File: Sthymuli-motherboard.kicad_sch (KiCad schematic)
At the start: 284 parts, among them J1 USB_C_Receptacle_USB2.0_16P, J2 Conn_01x09, J3 Conn_01x03, J4 Conn_01x06, Q1 Q_NMOS_Depletion_GSD, Q10 NX7002AK, Q11 NX7002AK, Q12 NX7002AK, Q13 NX7002AK, Q14 NX7002AK, Q15 NX7002AK, Q2 Q_NMOS_Depletion_GSD, Q3 Q_NMOS_Depletion_GSD, Q4 Q_NMOS_Depletion_GSD, Q5 Q_NMOS_Depletion_GSD, Q6 Q_NMOS_Depletion_GSD, Q7 PMOS, Q8 NX7002AK, Q9 NX7002AK, SW1 SW_Push, SW10 SW_Push, SW2 SW_Push, SW3 SW_Push, SW4 SW_Push, SW5 SW_Push, SW6 SW_Push, SW7 SW_Push, SW8 SW_Push, SW9 SW_Push, U1 ESP32-S3-WROOM-1, U10 74HC4051, U11 MCP6L01x-xOT, U12 74HC4051, U13 LSM6DS3, U14 LSM6DS3, U15 ITR9909, U16 ITR9909, U17 ITR9909, U18 ITR9909, U19 ITR9909, U2 AP2112K-3.3, U20 ITR9909, U21 ITR9909, U22 ITR9909, U3 BQ76905RGRR, U4 AP62300WU, U5 BQ25713, U6 AP62300WU, U7 MCP23017_SO, U8 AP22913CN4, U9 IRM-H6xxT

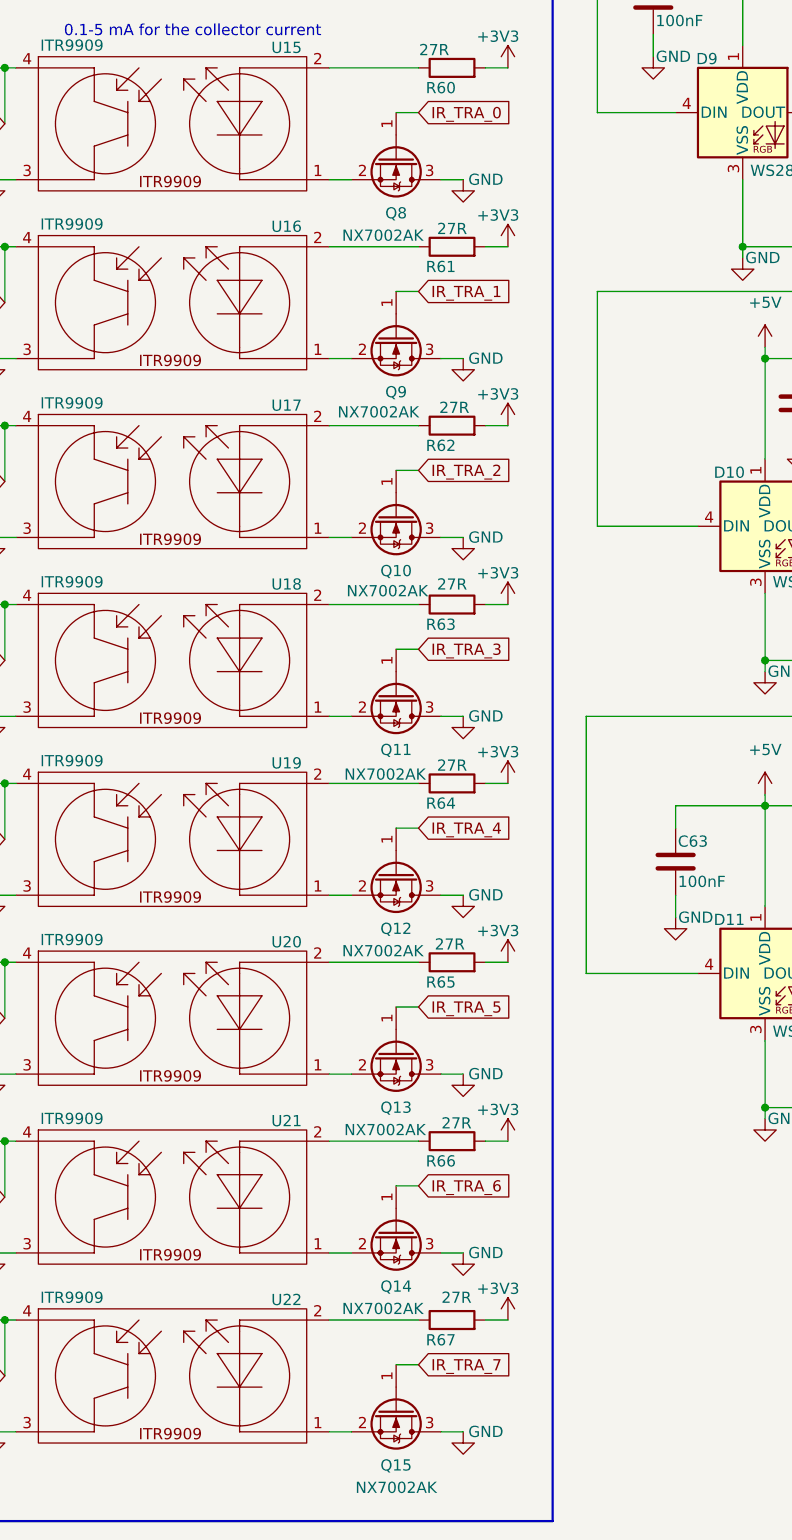
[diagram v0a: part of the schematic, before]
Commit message: added footprint
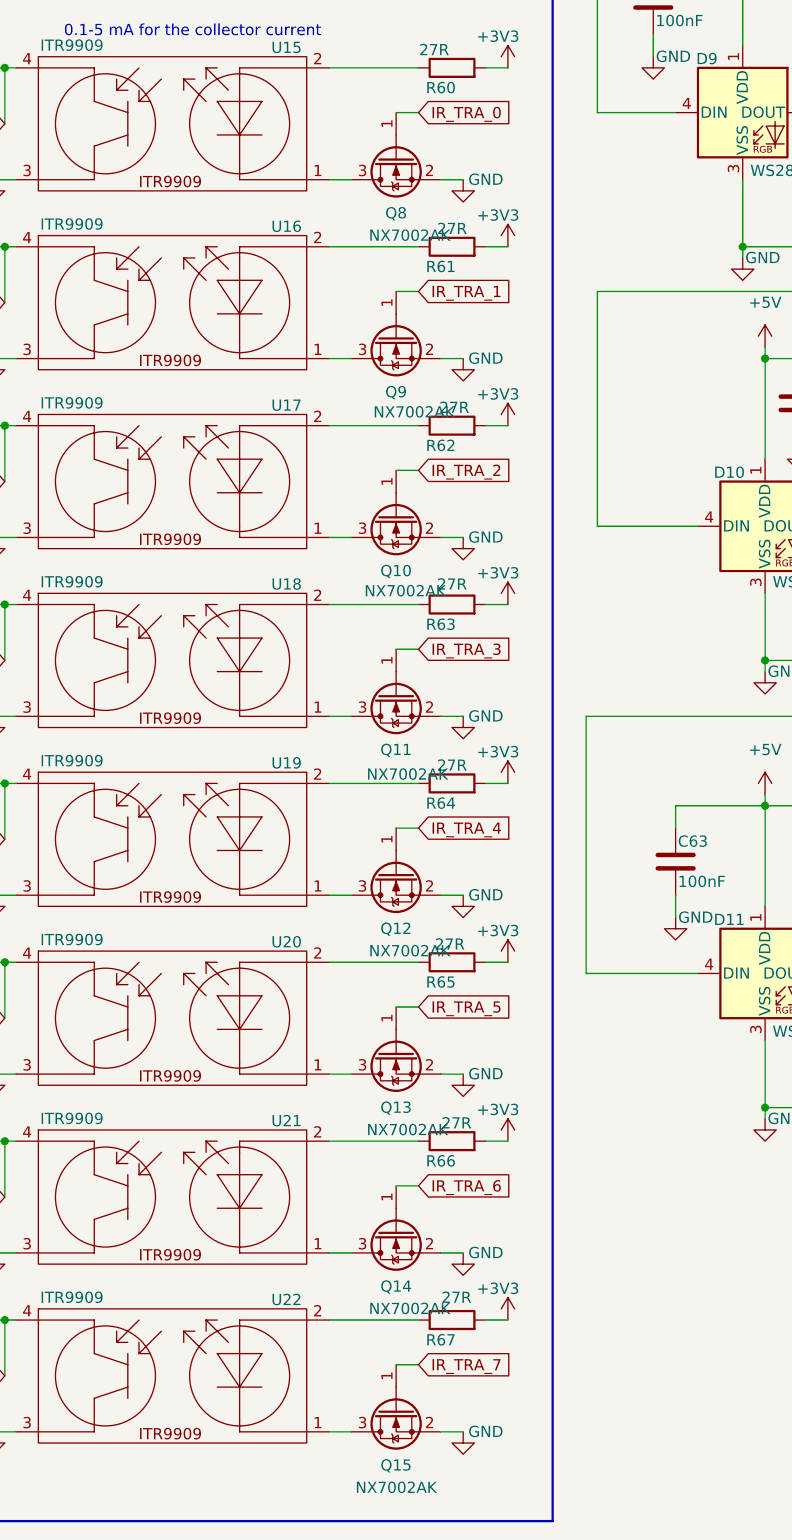
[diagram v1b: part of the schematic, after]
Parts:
- BT1, BT2, BT3, BT4: footprint (none) -> sthymuli:Battery_Holder_18650_robop
- D1, D12, D2, D3, D4, D5, D6: footprint (none) -> Diode_SMD:D_SOD-123F
- ES1: footprint (none) -> Package_DFN_QFN:QFN-28-1EP_4x4mm_P0.45mm_EP2.4x2.4mm
- F1, F2, F3, F4: footprint (none) -> Resistor_SMD:R_0805_2012Metric
- J1: footprint (none) -> Connector_USB:USB_C_Receptacle_G-Switch_GT-USB-7010ASV
- J2: footprint (none) -> Connector_PinHeader_2.54mm:PinHeader_1x09_P2.54mm_Vertical
- J3: footprint (none) -> Connector_PinHeader_2.54mm:PinHeader_1x03_P2.54mm_Vertical
- Q1, Q2, Q3, Q4, Q5, Q6, Q7: footprint (none) -> Package_SON:VSON-8_3.3x3.3mm_P0.65mm_NexFET
- Q10, Q11, Q12, Q13, Q14, Q15, Q8, Q9: footprint (none) -> Package_TO_SOT_SMD:SOT-23
- SW1, SW10, SW2, SW3, SW4, SW5, SW6, SW7, SW8, SW9: footprint (none) -> sthymuli:XKB5858
- TH1: footprint (none) -> Resistor_SMD:R_0603_1608Metric
- U15, U16, U17, U18: footprint (none) -> sthymuli:ITR_9909_Horizontal
- U19, U20, U21, U22: footprint (none) -> sthymuli:ITR_9909_Vertical
- U3: footprint BQ76905RGRR:IC_BQ76905RGRR -> Package_DFN_QFN:Texas_RGP0020H_VQFN-20-1EP_4x4mm_P0.5mm_EP2.4x2.4mm
- U5: footprint (none) -> Package_DFN_QFN:QFN-32-1EP_4x4mm_P0.4mm_EP2.9x2.9mm
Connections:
- net GND: now also Q10.2 (S), Q11.2 (S), Q12.2 (S), Q13.2 (S), Q14.2 (S), Q15.2 (S), Q8.2 (S), Q9.2 (S); no longer Q10.3 (D), Q11.3 (D), Q12.3 (D), Q13.3 (D), Q14.3 (D), Q15.3 (D), Q8.3 (D), Q9.3 (D)
- net at U16.1: now also Q9.3 (D); no longer Q9.2 (S)
- net at U20.1: now also Q13.3 (D); no longer Q13.2 (S)
- net at U22.1: now also Q15.3 (D); no longer Q15.2 (S)
- net at U15.1: now also Q8.3 (D); no longer Q8.2 (S)
- net at U18.1: now also Q11.3 (D); no longer Q11.2 (S)
- net at U21.1: now also Q14.3 (D); no longer Q14.2 (S)
- net at U17.1: now also Q10.3 (D); no longer Q10.2 (S)
- net at U19.1: now also Q12.3 (D); no longer Q12.2 (S)
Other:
- moved on the sheet: Q10, Q11, Q12, Q13, Q14, Q15, Q8, Q9

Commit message: started layout of component
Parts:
- removed C102, C63, C72, C78, C82, C86, C90, C96: 100nF, Capacitor_SMD:C_0402_1005Metric, symbol Device:C
- removed D11, D16, D20, D24, D28, D32, D36, D40: WS2812B, LED_SMD:LED_WS2812B_PLCC4_5.0x5.0mm_P3.2mm, symbol LED:WS2812B
- J4: footprint (none) -> sthymuli:ConnectorSpring
- L1: footprint (none) -> sthymuli:FHD4020S-2R2MT
- L2, L3: footprint (none) -> sthymuli:FXL0630-3R3-M
- L4: footprint (none) -> sthymuli:TDK VFS5045VA301
- LS1: footprint (none) -> sthymuli:Speaker KELIKING KLJ-01304T-08R07W
- MKTD4015BPN1: footprint (none) -> sthymuli:SAMZO MIC-4013-G-G00

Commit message: fixed some footprint issue, advanced layout
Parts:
- added C2: 100nF, Capacitor_SMD:C_0402_1005Metric, symbol Device:C
- added D2: WS2812B, LED_SMD:LED_WS2812B_PLCC4_5.0x5.0mm_P3.2mm, symbol LED:WS2812B
- C49: renamed from C27; footprint Capacitor_SMD:C_0402_1005Metric -> Capacitor_SMD:C_0805_2012Metric
- C50: renamed from C28; footprint Capacitor_SMD:C_0402_1005Metric -> Capacitor_SMD:C_0805_2012Metric
- C51: renamed from C29; footprint Capacitor_SMD:C_0402_1005Metric -> Capacitor_SMD:C_0805_2012Metric
- C72: renamed from C50; footprint Capacitor_SMD:C_0805_2012Metric -> Capacitor_SMD:C_0402_1005Metric
- C76: renamed from C54; footprint Capacitor_SMD:C_0805_2012Metric -> Capacitor_SMD:C_0402_1005Metric
- C81: renamed from C59; footprint Capacitor_SMD:C_0402_1005Metric -> Capacitor_SMD:C_0805_2012Metric
- renumbered C65 to C1, C62 to C10, C70 to C11, C76 to C12, C80 to C13, C84 to C14, C88 to C15, C94 to C16, C100 to C17, C68 to C18, C71 to C19, C77 to C20, C81 to C21, C85 to C22, C89 to C23, C95 to C24, C101 to C25, C4 to C26, C5 to C27, C6 to C28, C7 to C29, C74 to C3, C8 to C30, C9 to C31, C10 to C32, C11 to C33, C12 to C34, C13 to C35, C14 to C36, C15 to C37, C16 to C38, C17 to C39, C79 to C4, C18 to C40, C19 to C41, C20 to C42, C21 to C43, C22 to C44, C23 to C45, C24 to C46, C25 to C47, C26 to C48, C83 to C5, C30 to C52, C31 to C53, C32 to C54, C33 to C55, C34 to C56, C35 to C57, C36 to C58, C37 to C59, C87 to C6, C38 to C60, C39 to C61, C40 to C62, C41 to C63, C42 to C64, C43 to C65, C44 to C66, C45 to C67, C46 to C68, C47 to C69, C92 to C7, C48 to C70, C49 to C71, C51 to C73, C52 to C74, C53 to C75, C55 to C77, C56 to C78, C57 to C79, C98 to C8, C58 to C80, C60 to C82, C61 to C83, C64 to C84, C66 to C85, C67 to C86, C69 to C87, C73 to C88, C75 to C89, C104 to C9, C91 to C90, C93 to C91, C97 to C92, C99 to C93, C103 to C94, C105 to C95, C1 to C96, C2 to C97, C3 to C98, D13 to D1, D9 to D10, D14 to D11, D18 to D12, D22 to D13, D26 to D14, D30 to D15, D34 to D16, D38 to D17, D10 to D18, D15 to D19, D19 to D20, D23 to D21, D27 to D22, D31 to D23, D35 to D24, D39 to D25, D1 to D26, D2 to D27, D3 to D28, D4 to D29, D17 to D3, D5 to D30, D6 to D31, D7 to D32, D8 to D33, D12 to D34, D21 to D4, D25 to D5, D29 to D6, D33 to D7, D37 to D8, D41 to D9
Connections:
- net +5V: now also C2.1, D2.1 (VDD)
- net +BATT: now also D26.1 (K); no longer BT1.1 (+)
- net GND: now also C2.2, D2.3 (VSS)
- net at BT1.2 (-), D26.2 (A), F2.1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: now also D27.1 (K); no longer BT2.1 (+)
- net at BT2.2 (-), D27.2 (A), F3.1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: now also D28.1 (K); no longer BT3.1 (+)
- net at BT3.2 (-), D28.2 (A), F4.1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: now also D29.1 (K); no longer BT4.1 (+)
- net at F3.2: now also BT3.1 (+); no longer D28.1 (K)
- net at F2.2: now also BT2.1 (+); no longer D27.1 (K)
- net at F1.2: now also BT1.1 (+); no longer D26.1 (K)
- net at D3.4 (DIN): now also D2.2 (DOUT); no longer D1.2 (DOUT)
- net at F4.2: now also BT4.1 (+); no longer D29.1 (K)
- new net: D1.2 (DOUT), D2.4 (DIN)
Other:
- note added: "25 RGB LEDs 4 side with 6 led IR proximity 1 Battery status"
- note removed: "32 RGB LEDs 4 side IR proximity 6*4 led per capacitive buttons 4 center led for the button"
- moved on the sheet: C1, C10, C11, C12, C13, C14, C15, C16, C17, C18, C19, C20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
